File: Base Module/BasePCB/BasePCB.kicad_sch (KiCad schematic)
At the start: 146 parts, among them J1 USB_A, J2 Conn_01x05_Female, J3 Conn_01x05_Male, J4 Conn_01x05_Female, J5 Conn_01x05_Female, SW1 SW_Push, U1 ATmega32U4-A, Y1 Crystal_GND24_Small

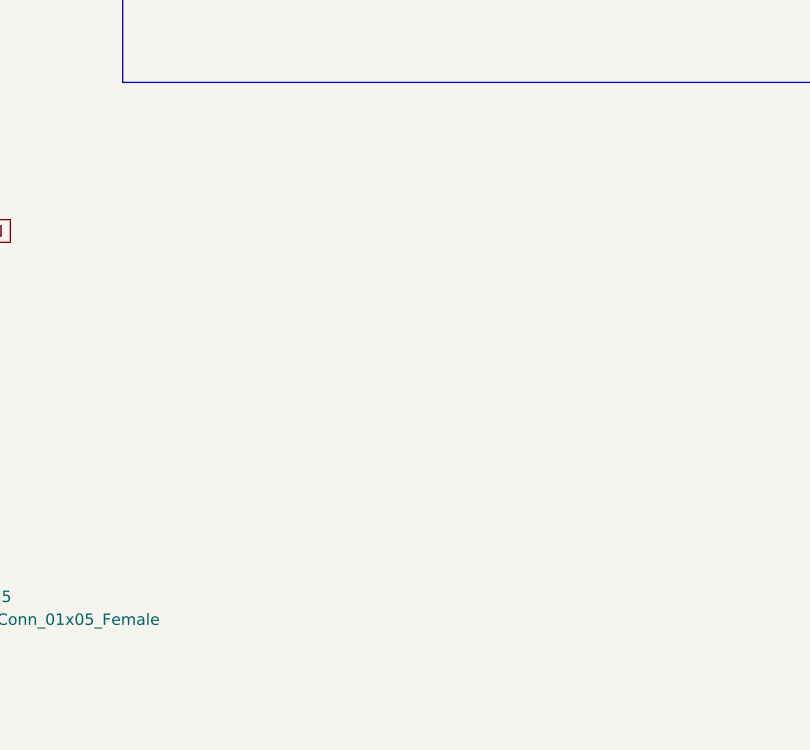
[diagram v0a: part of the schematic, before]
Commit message: Added potential new connectors
might use them or not idfk bro
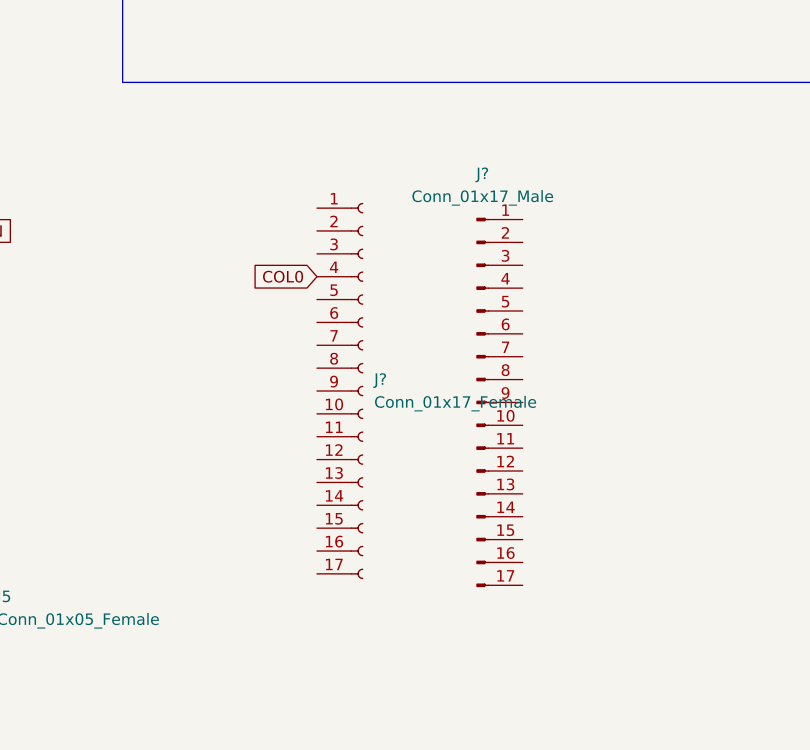
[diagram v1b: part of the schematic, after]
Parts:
- added J?: Conn_01x17_Male, symbol Connector:Conn_01x17_Male
- added J?: Conn_01x17_Female, symbol Connector:Conn_01x17_Female
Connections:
- net COL0: now also J?.4 (Pin_4)
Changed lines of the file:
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@@
     )
   )
+  (global_label "COL0" (shape input) (at 148.59 210.82 180) (fields_autoplaced)
+    (effects (font (size 1.27 1.27)) (justify right))
+    (property "Intersheet References" "${INTERSHEET_REFS}" (id 0) (at 141.3388 210.7406 0)
+      (effects (font (size 1.27 1.27)) (justify right) hide)
+    )
+  )
   (global_label "ROW3" (shape input) (at 149.86 148.59 180) (fields_autoplaced)
     (effects (font (size 1.27 1.27)) (justify right))
@@
     (pin "5")
   )
+  (symbol (lib_id "Connector:Conn_01x17_Male") (at 166.37 224.79 0) (unit 1)
+    (in_bom yes) (on_board yes) (fields_autoplaced)
+    (property "Reference" "J?" (id 0) (at 167.005 199.39 0))
+    (property "Value" "Conn_01x17_Male" (id 1) (at 167.005 201.93 0))
+    (property "Footprint" "" (id 2) (at 166.37 224.79 0)
+      (effects (font (size 1.27 1.27)) hide)
+    )
+    (property "Datasheet" "~" (id 3) (at 166.37 224.79 0)
+      (effects (font (size 1.27 1.27)) hide)
+    )
+    (pin "1")
+    (pin "10")
+    (pin "11")
+    (pin "12")
+    (pin "13")
+    (pin "14")
+    (pin "15")
+    (pin "16")
+    (pin "17")
+    (pin "2")
+    (pin "3")
+    (pin "4")
+    (pin "5")
+    (pin "6")
+    (pin "7")
+    (pin "8")
+    (pin "9")
+  )
   (symbol (lib_id "Device:D_Small") (at 353.06 146.05 90) (unit 1)
     (in_bom yes) (on_board yes) (fields_autoplaced)
@@
     (pin "1")
   )
+  (symbol (lib_id "Connector:Conn_01x17_Female") (at 153.67 223.52 0) (unit 1)
+    (in_bom yes) (on_board yes) (fields_autoplaced)
+    (property "Reference" "J?" (id 0) (at 154.94 222.2499 0)
+      (effects (font (size 1.27 1.27)) (justify left))
+    )
+    (property "Value" "Conn_01x17_Female" (id 1) (at 154.94 224.7899 0)
+      (effects (font (size 1.27 1.27)) (justify left))
+    )
+    (property "Footprint" "" (id 2) (at 153.67 223.52 0)
+      (effects (font (size 1.27 1.27)) hide)
+    )
+    (property "Datasheet" "~" (id 3) (at 153.67 223.52 0)
+      (effects (font (size 1.27 1.27)) hide)
+    )
+    (pin "1")
+    (pin "10")
+    (pin "11")
+    (pin "12")
+    (pin "13")
+    (pin "14")
+    (pin "15")
+    (pin "16")
+    (pin "17")
+    (pin "2")
+    (pin "3")
+    (pin "4")
+    (pin "5")
+    (pin "6")
+    (pin "7")
+    (pin "8")
+    (pin "9")
+  )
   (symbol (lib_id "Device:R_Small") (at 53.34 83.82 90) (unit 1)
     (in_bom yes) (on_board yes) (fields_autoplaced)
@@
       (reference "J5") (unit 1) (value "Conn_01x05_Female") (footprint "Connector_JST:JST_PH_S5B-PH-K_1x05_P2.00mm_Horizontal")
     )
+    (path "/7f4b871e-b6b9-40d4-960c-7c0aa6791a72"
+      (reference "J?") (unit 1) (value "Conn_01x17_Male") (footprint "")
+    )
+    (path "/90d46ba0-9667-4cbc-8ba4-f7cc374719c5"
+      (reference "J?") (unit 1) (value "Conn_01x17_Female") (footprint "")
+    )
     (path "/dad534c2-e236-4d66-a9ff-bc0c560250c3"

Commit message: Revert "Added potential new connectors"
This reverts commit 86ebb0b8c096f4d7f87798976226ac9f3014035e.
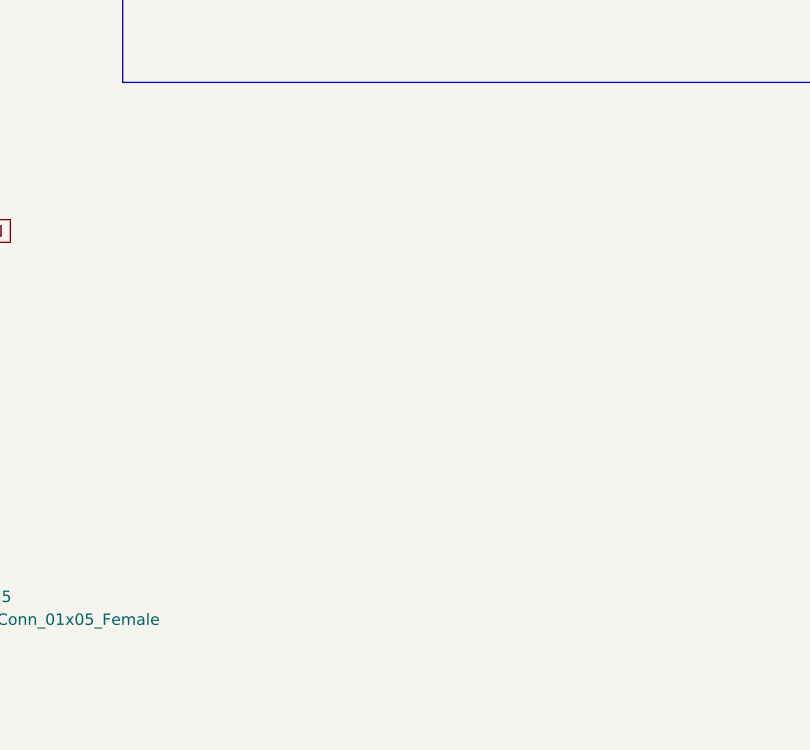
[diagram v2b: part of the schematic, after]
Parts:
- removed J?: Conn_01x17_Male, symbol Connector:Conn_01x17_Male
- removed J?: Conn_01x17_Female, symbol Connector:Conn_01x17_Female
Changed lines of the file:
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@@
     )
   )
-  (global_label "COL0" (shape input) (at 148.59 210.82 180) (fields_autoplaced)
-    (effects (font (size 1.27 1.27)) (justify right))
-    (property "Intersheet References" "${INTERSHEET_REFS}" (id 0) (at 141.3388 210.7406 0)
-      (effects (font (size 1.27 1.27)) (justify right) hide)
-    )
-  )
   (global_label "ROW3" (shape input) (at 149.86 148.59 180) (fields_autoplaced)
     (effects (font (size 1.27 1.27)) (justify right))
@@
     (pin "5")
   )
-  (symbol (lib_id "Connector:Conn_01x17_Male") (at 166.37 224.79 0) (unit 1)
-    (in_bom yes) (on_board yes) (fields_autoplaced)
-    (property "Reference" "J?" (id 0) (at 167.005 199.39 0))
-    (property "Value" "Conn_01x17_Male" (id 1) (at 167.005 201.93 0))
-    (property "Footprint" "" (id 2) (at 166.37 224.79 0)
-      (effects (font (size 1.27 1.27)) hide)
-    )
-    (property "Datasheet" "~" (id 3) (at 166.37 224.79 0)
-      (effects (font (size 1.27 1.27)) hide)
-    )
-    (pin "1")
-    (pin "10")
-    (pin "11")
-    (pin "12")
-    (pin "13")
-    (pin "14")
-    (pin "15")
-    (pin "16")
-    (pin "17")
-    (pin "2")
-    (pin "3")
-    (pin "4")
-    (pin "5")
-    (pin "6")
-    (pin "7")
-    (pin "8")
-    (pin "9")
-  )
   (symbol (lib_id "Device:D_Small") (at 353.06 146.05 90) (unit 1)
     (in_bom yes) (on_board yes) (fields_autoplaced)
@@
     (pin "1")
   )
-  (symbol (lib_id "Connector:Conn_01x17_Female") (at 153.67 223.52 0) (unit 1)
-    (in_bom yes) (on_board yes) (fields_autoplaced)
-    (property "Reference" "J?" (id 0) (at 154.94 222.2499 0)
-      (effects (font (size 1.27 1.27)) (justify left))
-    )
-    (property "Value" "Conn_01x17_Female" (id 1) (at 154.94 224.7899 0)
-      (effects (font (size 1.27 1.27)) (justify left))
-    )
-    (property "Footprint" "" (id 2) (at 153.67 223.52 0)
-      (effects (font (size 1.27 1.27)) hide)
-    )
-    (property "Datasheet" "~" (id 3) (at 153.67 223.52 0)
-      (effects (font (size 1.27 1.27)) hide)
-    )
-    (pin "1")
-    (pin "10")
-    (pin "11")
-    (pin "12")
-    (pin "13")
-    (pin "14")
-    (pin "15")
-    (pin "16")
-    (pin "17")
-    (pin "2")
-    (pin "3")
-    (pin "4")
-    (pin "5")
-    (pin "6")
-    (pin "7")
-    (pin "8")
-    (pin "9")
-  )
   (symbol (lib_id "Device:R_Small") (at 53.34 83.82 90) (unit 1)
     (in_bom yes) (on_board yes) (fields_autoplaced)
@@
       (reference "J5") (unit 1) (value "Conn_01x05_Female") (footprint "Connector_JST:JST_PH_S5B-PH-K_1x05_P2.00mm_Horizontal")
     )
-    (path "/7f4b871e-b6b9-40d4-960c-7c0aa6791a72"
-      (reference "J?") (unit 1) (value "Conn_01x17_Male") (footprint "")
-    )
-    (path "/90d46ba0-9667-4cbc-8ba4-f7cc374719c5"
-      (reference "J?") (unit 1) (value "Conn_01x17_Female") (footprint "")
-    )
     (path "/dad534c2-e236-4d66-a9ff-bc0c560250c3"
